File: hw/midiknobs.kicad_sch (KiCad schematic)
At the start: 35 parts, among them J1 AVR-ISP, J2 MIDI out, Q1 2N7000, SW1 rotary, SW2 button, SW3 button, SW4 button, SW5 button, SW6 Channel, U1 ATmega168-20P, U2 MAX232, Y1 4MHz

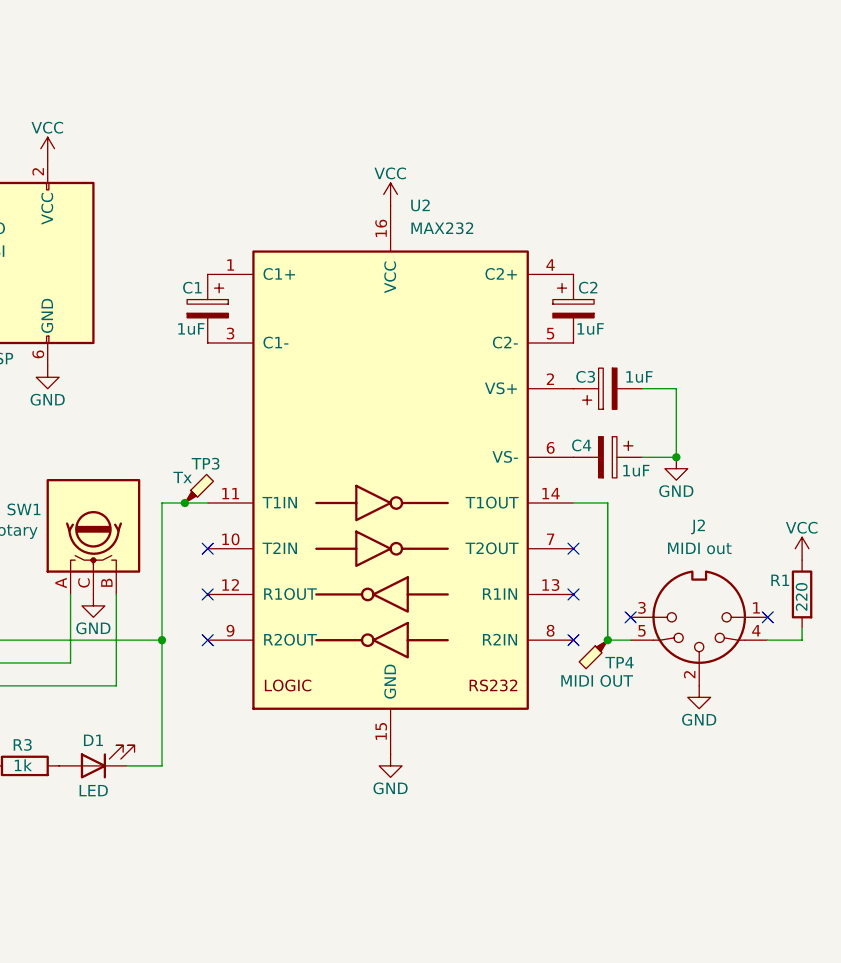
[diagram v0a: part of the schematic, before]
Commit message: rotary encoder
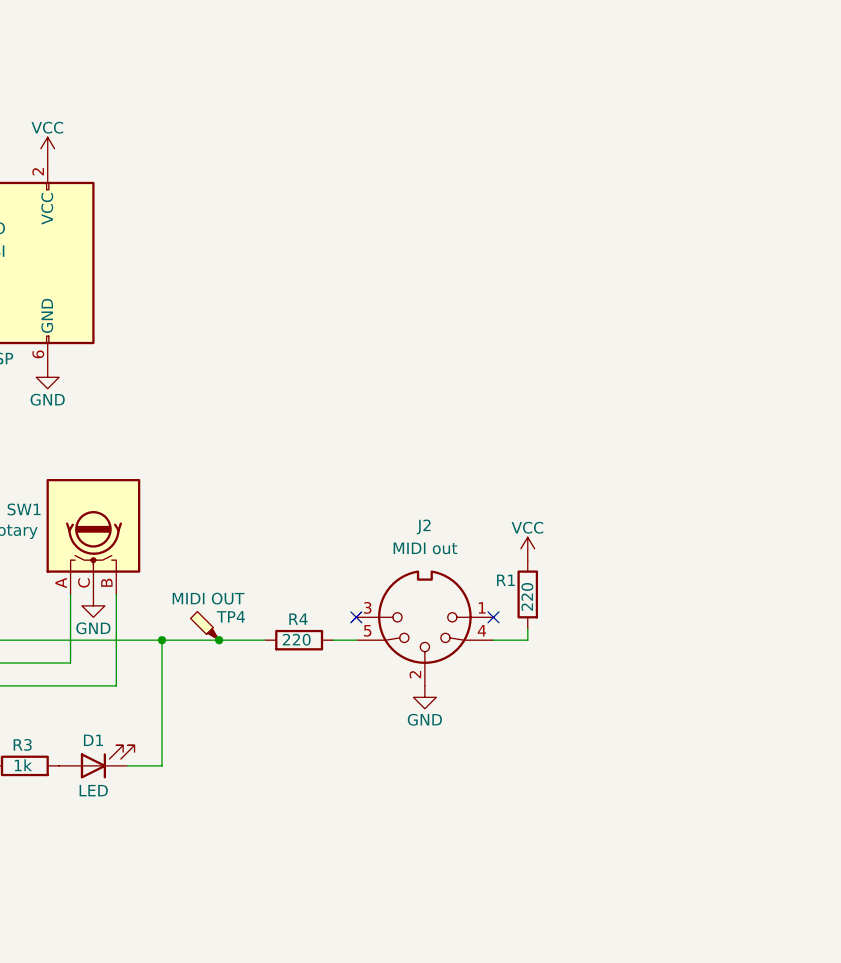
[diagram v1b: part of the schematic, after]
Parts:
- removed C1, C2, C3, C4: 1uF, symbol Device:C_Polarized
- removed TP3: Tx, symbol Connector:TestPoint_Probe
- removed U2: MAX232, symbol Interface_UART:MAX232
- added R4: 220, symbol Device:R
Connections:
- net at D1.1 (K), U1.3 (PD1): now also TP4.1, R4.2
- net at J2.5: now also R4.1; no longer TP4.1
- no-connect marks 10 -> 4
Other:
- moved on the sheet: J2, R1, TP4
